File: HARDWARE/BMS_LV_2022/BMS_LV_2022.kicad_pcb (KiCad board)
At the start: 4 copper layers, 90 x 45 mm, 159 parts, among them J1 Conn_01x06_Male, J11 Conn_01x07_Female, J12 Conn_01x08_Female, J2 Conn_01x12_Male, J3 USB_B_Mini, J4 Battery+, J5 Battery-, Q1 BC846, Q10 BSS138, Q11 SiSS05DN, Q12 SiSS05DN, Q2 Q_NMOS_GSD, Q3 Q_NMOS_GSD, Q4 Q_NMOS_GSD, Q5 Q_NMOS_GSD, Q6 Q_NMOS_GSD, Q7 Q_NMOS_GSD, Q8 SiSS05DN, Q9 SiSS05DN, SW1 SW_Push, U1 STM32L4P5RET6, U2 LD3985M33R_TSOT23, U3 LMR23610, U4 ATA6561-GAQW-N, U5 ACHS-7123, Y1 Crystal

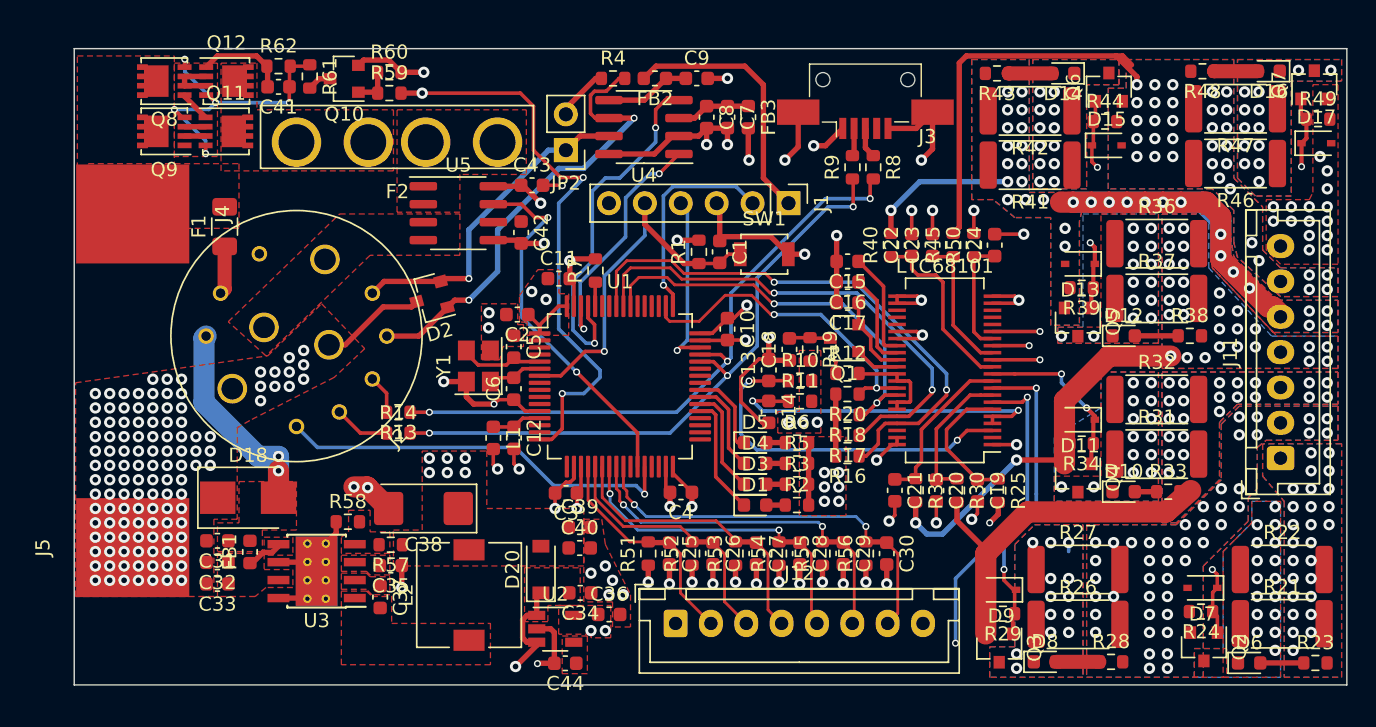
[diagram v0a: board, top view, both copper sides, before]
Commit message: Small bug fixes
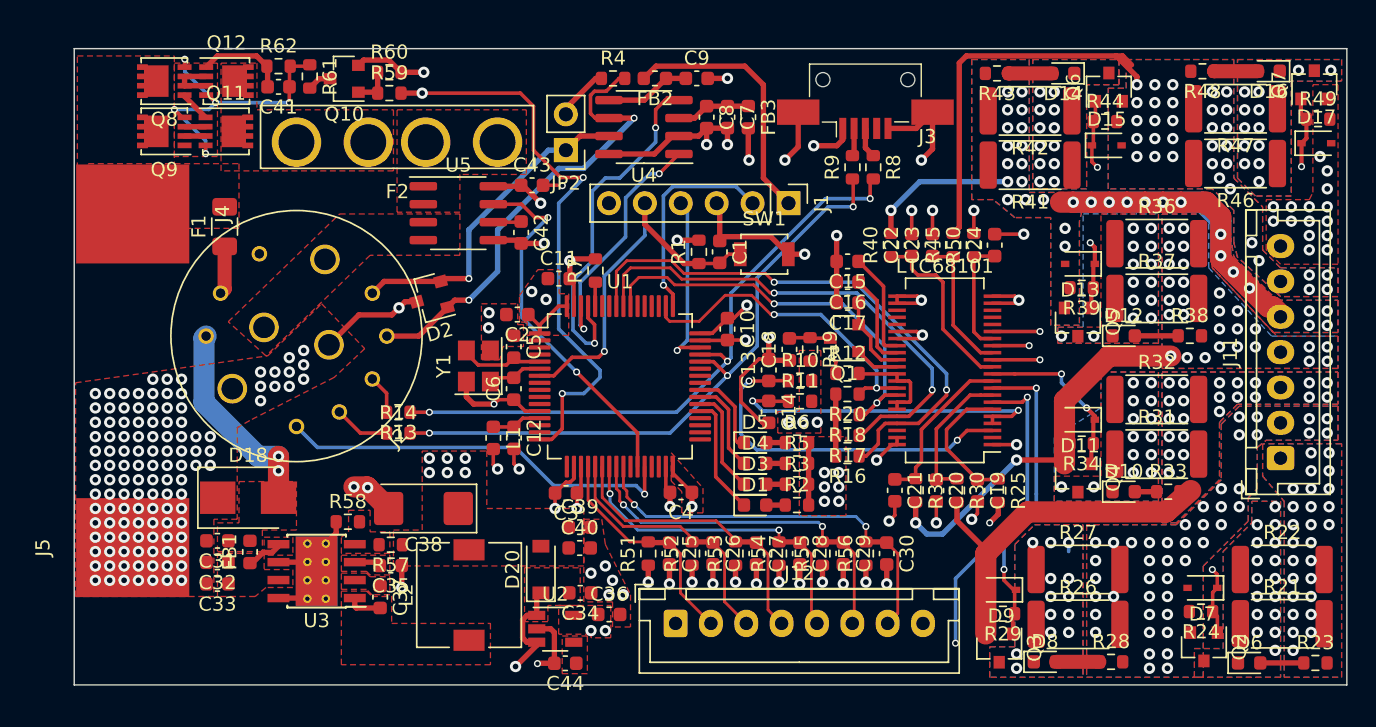
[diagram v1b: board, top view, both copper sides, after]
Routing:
- net Net-(C37-Pad2): track 0.00 -> 2.43 mm
- net Net-(C42-Pad1): track 0.00 -> 1.98 mm
- net Net-(C35-Pad2): track 0.00 -> 1.87 mm
- net GND: track 100.6 -> 99.0 mm
- net +5VD: track 88.0 -> 89.4 mm
